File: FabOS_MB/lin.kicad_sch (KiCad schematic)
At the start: 7 parts, among them J3 USB_A, U7 NCV7329

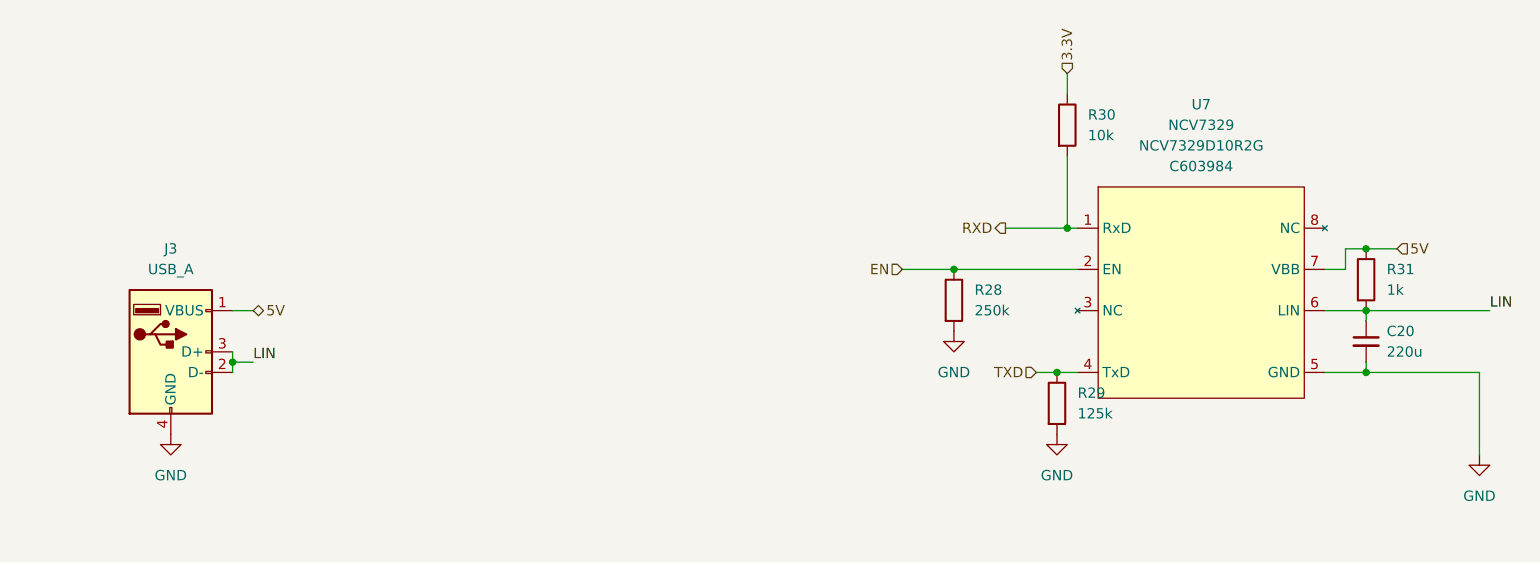
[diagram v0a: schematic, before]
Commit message: update pcb
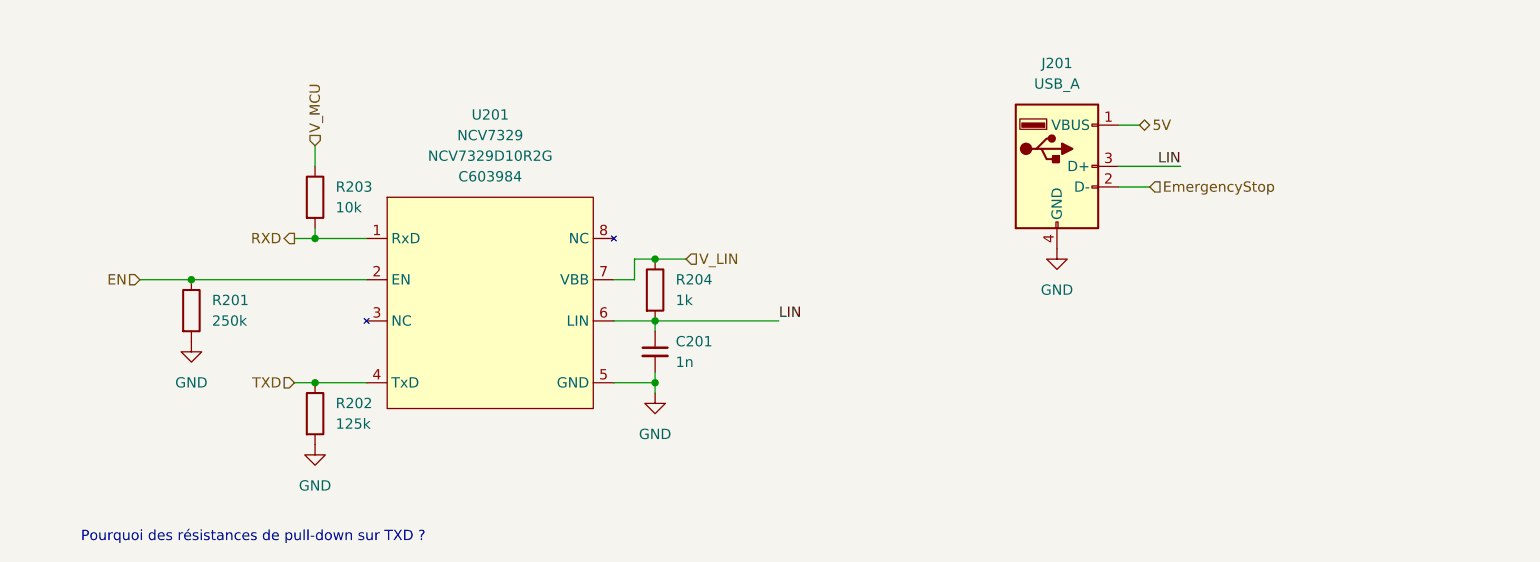
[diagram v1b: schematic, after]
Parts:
- C201: renamed from C20; value 220u -> 1n
- renumbered J3 to J201, R28 to R201, R29 to R202, R30 to R203, R31 to R204, U7 to U201
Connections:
- net 5V: no longer R204.1, U201.7 (VBB)
- net LIN: no longer J201.2 (D-)
- net 3.3V renamed V_MCU
- new net EmergencyStop: J201.2 (D-)
- new net V_LIN: R204.1, U201.7 (VBB)
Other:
- note added: "Pourquoi des résistances de pull-down sur TXD ?"
- moved on the sheet: C201, J201, R201, R202, R203, R204, U201
